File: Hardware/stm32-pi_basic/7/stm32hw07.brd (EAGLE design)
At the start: 71.5 x 74 mm, 75 parts, among them IC1 CP2102, J1 CONN_12X2, U1 ESP32-WROOM-32D

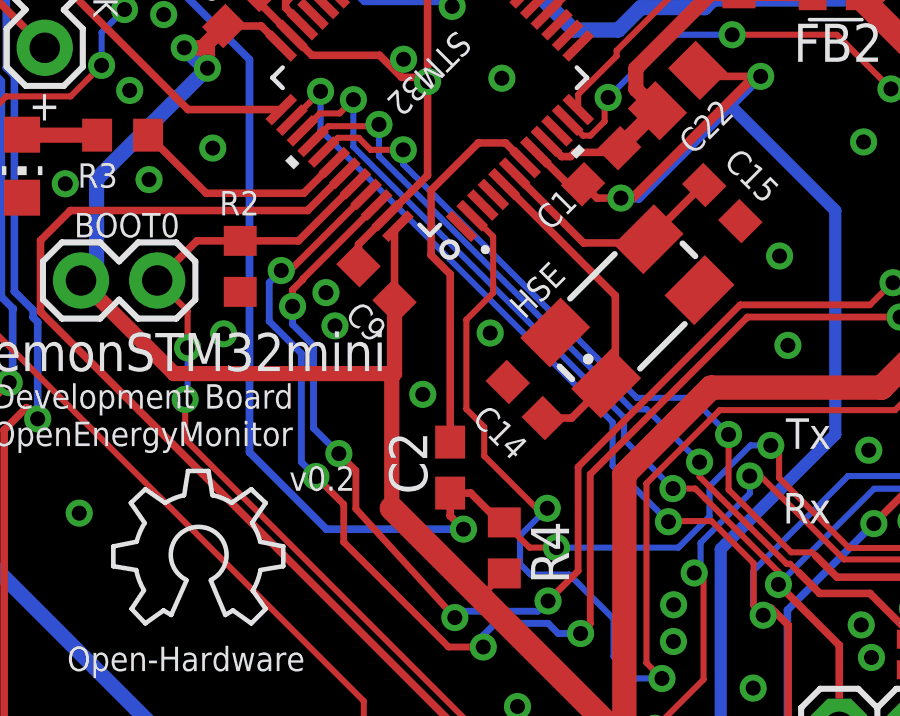
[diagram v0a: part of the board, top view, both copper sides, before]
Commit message: sync
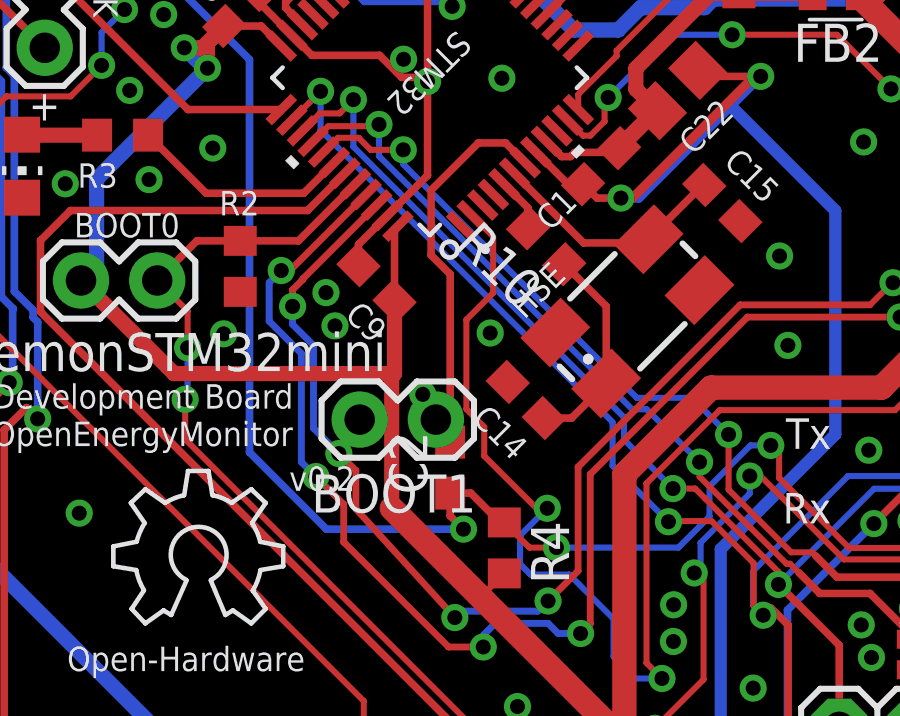
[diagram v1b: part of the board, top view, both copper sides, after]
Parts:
- added BOOT1: (no value), SparkFun:1X02
- added R10: 10k, resistor:R0603
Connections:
- removed net LSE_IN: STM32.3
- removed net LSE_OUT: STM32.4
- new net HSE_IN_: C14.1, HSE.1, R10.1
- net GND: now also BOOT1.2
- net HSE_IN: now also R10.2; no longer C14.1, HSE.1
- net NRST: now also BOOT1.1
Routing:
- net HSE_IN: track 10.9 -> 2.40 mm
- net HSE_IN_: track 0.00 -> 7.11 mm

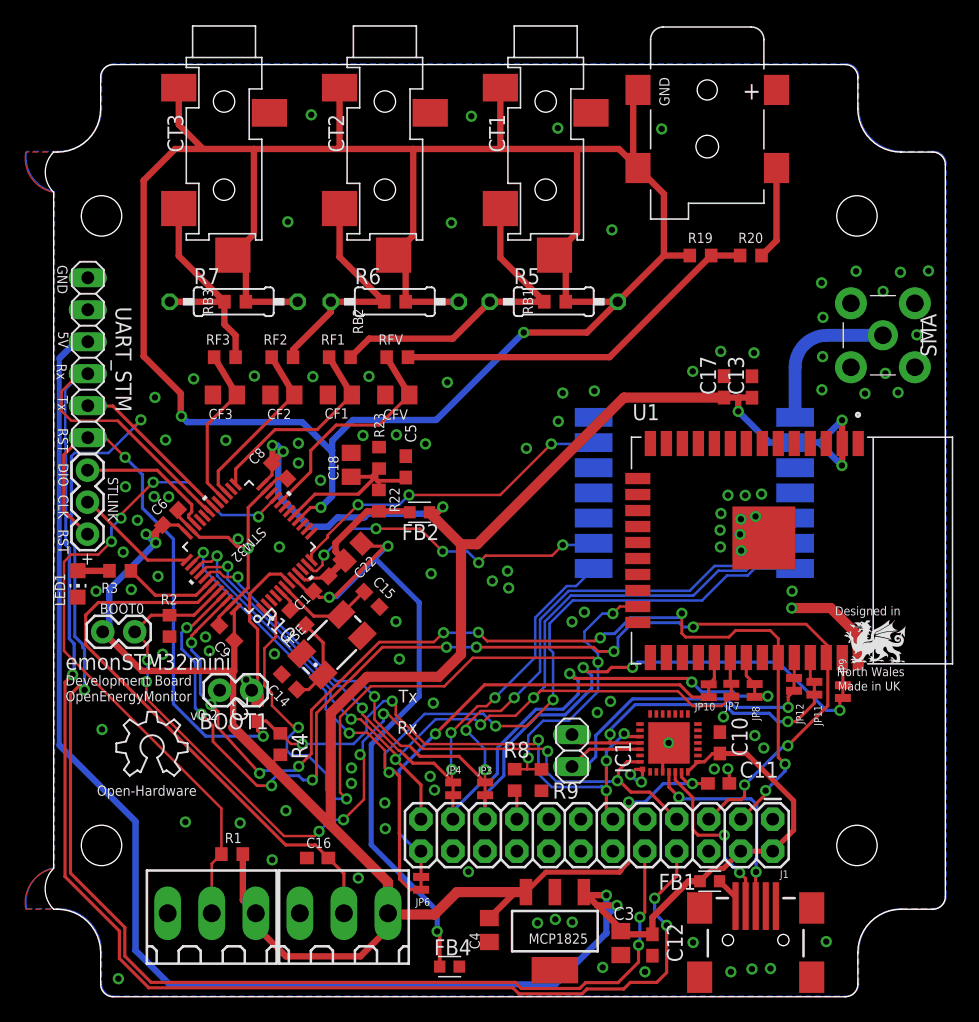
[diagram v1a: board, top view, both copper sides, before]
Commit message: sync, raido tested
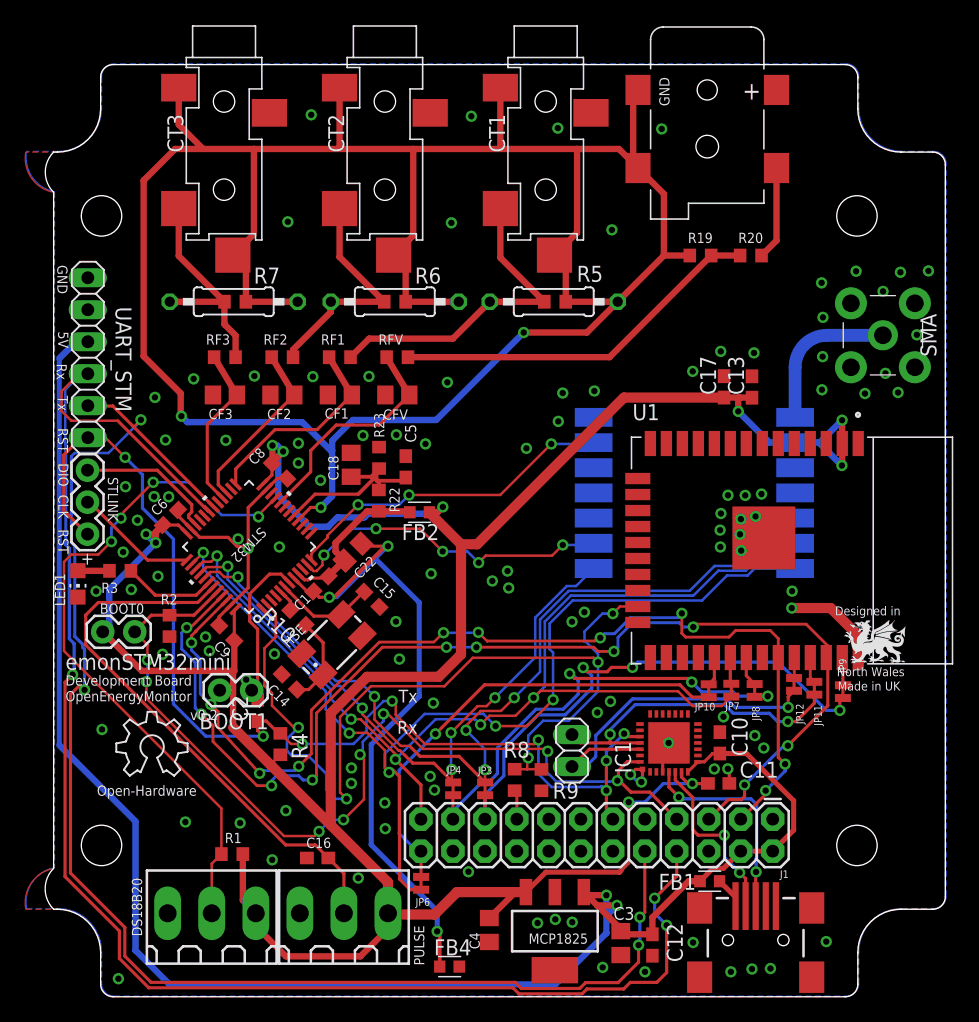
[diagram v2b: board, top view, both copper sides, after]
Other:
- board text added: "PULSE"
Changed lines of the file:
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@@
 <layer number="14" name="Route14" color="1" fill="6" visible="no" active="no"/>
 <layer number="15" name="Route15" color="4" fill="6" visible="no" active="no"/>
-<layer number="16" name="Bottom" color="1" fill="1" visible="yes" active="yes"/>
+<layer number="16" name="Bottom" color="1" fill="1" visible="no" active="yes"/>
 <layer number="17" name="Pads" color="2" fill="1" visible="yes" active="yes"/>
 <layer number="18" name="Vias" color="2" fill="1" visible="yes" active="yes"/>
@@
 <layer number="110" name="fp0" color="7" fill="1" visible="no" active="yes"/>
 <layer number="111" name="LPC17xx" color="7" fill="1" visible="no" active="yes"/>
-<layer number="112" name="tSilk" color="7" fill="1" visible="yes" active="yes"/>
+<layer number="112" name="tSilk" color="7" fill="1" visible="no" active="yes"/>
 <layer number="113" name="IDFDebug" color="4" fill="1" visible="no" active="yes"/>
 <layer number="114" name="Route14" color="7" fill="1" visible="no" active="no"/>
@@
 <wire x1="43.482753125" y1="53.1352625" x2="42.738803125" y2="51.339209375" width="0.508" layer="42" curve="45.00007"/>
 <wire x1="42.738803125" y1="51.339209375" x2="42.738803125" y2="48.560228125" width="0.508" layer="42"/>
+<text x="36.953365625" y="8.771184375" size="0.8128" layer="21" font="vector" ratio="20" rot="R90">PULSE</text>
+<text x="13.727" y="15.73270625" size="0.8128" layer="21" font="vector" ratio="20" rot="R270">DS18B20</text>
 </plain>
 <attributes>
@@
 <attribute name="NAME" x="42.095746875" y="76.3895" size="1.27" layer="25" rot="R270"/>
 </element>
-<element name="RB1" library="resistor" package="R0603" value="22r" x="47.33749375" y="61.487934375" smashed="yes">
-<attribute name="NAME" x="45.58749375" y="60.487934375" size="0.8128" layer="25" font="vector" ratio="20" rot="R90"/>
-</element>
+<element name="RB1" library="resistor" package="R0603" value="22r" x="47.33749375" y="61.487934375" smashed="yes"/>
 <element name="RF1" library="resistor" package="R0603" value="9k1" x="30.245315625" y="57.08205625" smashed="yes" rot="R180">
 <attribute name="NAME" x="28.745315625" y="58.08205625" size="0.8128" layer="25" font="vector" ratio="20"/>
@@
 <attribute name="NAME" x="29.322746875" y="76.3895" size="1.27" layer="25" rot="R270"/>
 </element>
-<element name="RB2" library="resistor" package="R0603" value="6R8" x="34.622996875" y="61.487934375" smashed="yes">
-<attribute name="NAME" x="32.0911875" y="58.923040625" size="0.8128" layer="25" font="vector" ratio="20" rot="R90"/>
-</element>
+<element name="RB2" library="resistor" package="R0603" value="6R8" x="34.622996875" y="61.487934375" smashed="yes"/>
 <element name="RF2" library="resistor" package="R0603" value="9k1" x="25.67895" y="57.08205625" smashed="yes" rot="R180">
 <attribute name="NAME" x="24.17895" y="58.08205625" size="0.8128" layer="25" font="vector" ratio="20"/>
@@
 <attribute name="NAME" x="16.549746875" y="76.3895" size="1.27" layer="25" rot="R270"/>
 </element>
-<element name="RB3" library="resistor" package="R0603" value="6R8" x="21.933640625" y="61.487934375" smashed="yes">
-<attribute name="NAME" x="20.183640625" y="60.487934375" size="0.8128" layer="25" font="vector" ratio="20" rot="R90"/>
-</element>
+<element name="RB3" library="resistor" package="R0603" value="6R8" x="21.933640625" y="61.487934375" smashed="yes"/>
 <element name="RF3" library="resistor" package="R0603" value="9k1" x="21.112584375" y="57.08205625" smashed="yes" rot="R180">
 <attribute name="NAME" x="19.612584375" y="58.08205625" size="0.8128" layer="25" font="vector" ratio="20"/>
@@
 </element>
 <element name="R5" library="rcl" library_urn="urn:adsk.eagle:library:334" package="0207/10" package3d_urn="urn:adsk.eagle:package:23491/2" value="" x="47.23638125" y="61.487934375" smashed="yes">
-<attribute name="NAME" x="44.06138125" y="62.884934375" size="1.27" layer="25" ratio="10"/>
+<attribute name="NAME" x="49.064675" y="63.070353125" size="1.27" layer="25" ratio="10"/>
 <attribute name="POPULARITY" value="81" x="47.23638125" y="61.487934375" size="1.778" layer="27" display="off"/>
 <attribute name="SPICEPREFIX" value="R" x="47.23638125" y="61.487934375" size="1.778" layer="27" display="off"/>
@@
 </element>
 <element name="R6" library="rcl" library_urn="urn:adsk.eagle:library:334" package="0207/10" package3d_urn="urn:adsk.eagle:package:23491/2" value="" x="34.610553125" y="61.487934375" smashed="yes">
-<attribute name="NAME" x="31.435553125" y="62.884934375" size="1.27" layer="25" ratio="10"/>
+<attribute name="NAME" x="36.207196875" y="62.9311625" size="1.27" layer="25" ratio="10"/>
 <attribute name="POPULARITY" value="81" x="34.610553125" y="61.487934375" size="1.778" layer="27" display="off"/>
 <attribute name="SPICEPREFIX" value="R" x="34.610553125" y="61.487934375" size="1.778" layer="27" display="off"/>
@@
 </element>
 <element name="R7" library="rcl" library_urn="urn:adsk.eagle:library:334" package="0207/10" package3d_urn="urn:adsk.eagle:package:23491/2" value="" x="21.814540625" y="61.487934375" smashed="yes">
-<attribute name="NAME" x="18.639540625" y="62.884934375" size="1.27" layer="25" ratio="10"/>
+<attribute name="NAME" x="23.411184375" y="62.9311625" size="1.27" layer="25" ratio="10"/>
 <attribute name="POPULARITY" value="81" x="21.814540625" y="61.487934375" size="1.778" layer="27" display="off"/>
 <attribute name="SPICEPREFIX" value="R" x="21.814540625" y="61.487934375" size="1.778" layer="27" display="off"/>

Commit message: sync
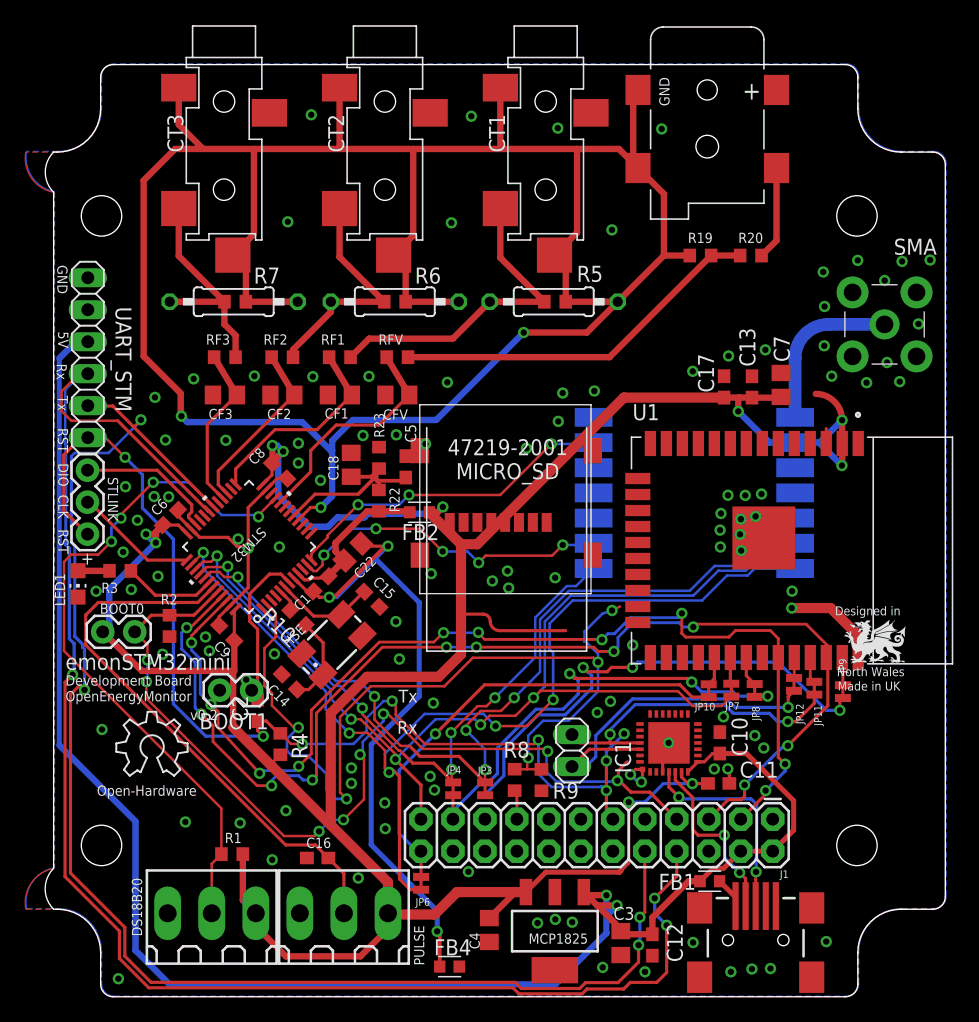
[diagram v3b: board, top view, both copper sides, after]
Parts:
- added C7: 22uF, rcl:C0805
- added U$3: 47219-2001_MICROSD, MOLEX 47219-2001:47219-2001_MICROSD
- moved SMA 0.87 mm to (73.5, 59.7)
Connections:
- new net MICROSD_CS: U$3.PIN2, U1.16
- net +3V3: now also C7.1, U$3.PIN4
- net BOOT0: no longer IC1.28
- net ESP_BOOT0: now also IC1.23
- net ESP_CLK: now also U$3.PIN5
- net ESP_MISO: now also U$3.PIN7
- net ESP_MOSI: now also U$3.PIN3
- net ESP_RST: now also IC1.24
- net GND: now also C7.2, U$3.P$1, U$3.P$2, U$3.P$3, U$3.P$4, U$3.PIN6
- net RPI_CONNECTED: now also U1.13; no longer U1.23
- net RPI_MISO: now also JP3.2; no longer JP4.2
- net RPI_MOSI: now also JP4.2; no longer JP3.2
- net RST_STM: no longer IC1.24
- net STM_RX: now also U1.28
- net STM_TX: now also U1.27
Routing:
- net +3V3: track 219.4 -> 233.9 mm
- net RPI_MOSI: track 42.5 -> 38.7 mm
- net RPI_CONNECTED: track 72.5 -> 71.0 mm
- net ESP_RST: track 0.00 -> 1.18 mm
- net RST_STM: track 88.6 -> 87.6 mm
- net BOOT0: track 75.2 -> 74.2 mm
- net N$18: track 12.0 -> 12.9 mm
